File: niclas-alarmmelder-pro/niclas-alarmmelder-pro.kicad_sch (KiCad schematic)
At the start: 16 parts, among them J1 DIN-5_180degree, SW1 SW_SPST, U1 MOUDLE-SEEEDUINO-XIAO-ESP32C3, U2 TME-0503S

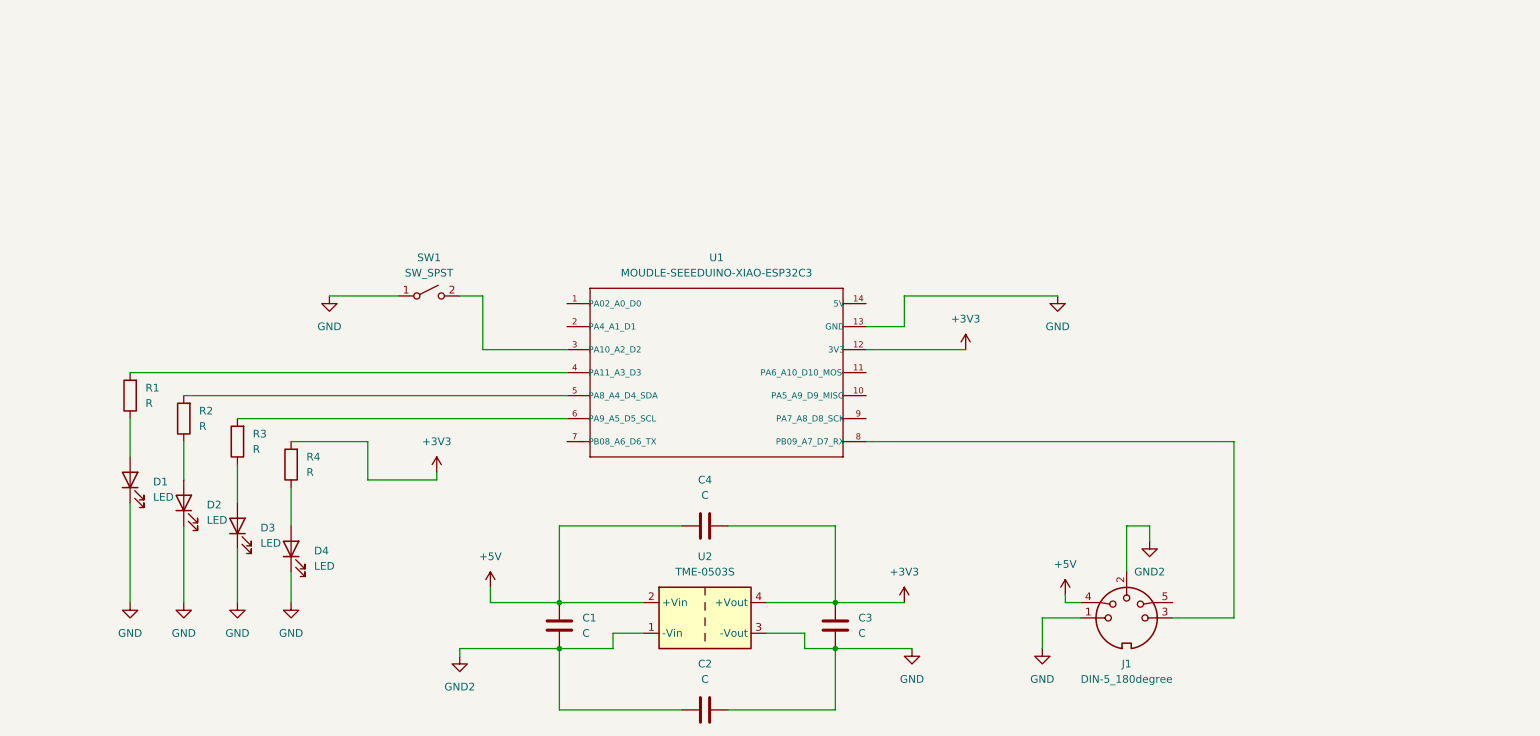
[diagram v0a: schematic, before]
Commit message: release ready
Sollte so funktionieren, eine Schraube mag oder mag nicht accessible sein je nach Schalter aber idc worst case reichen auch 2
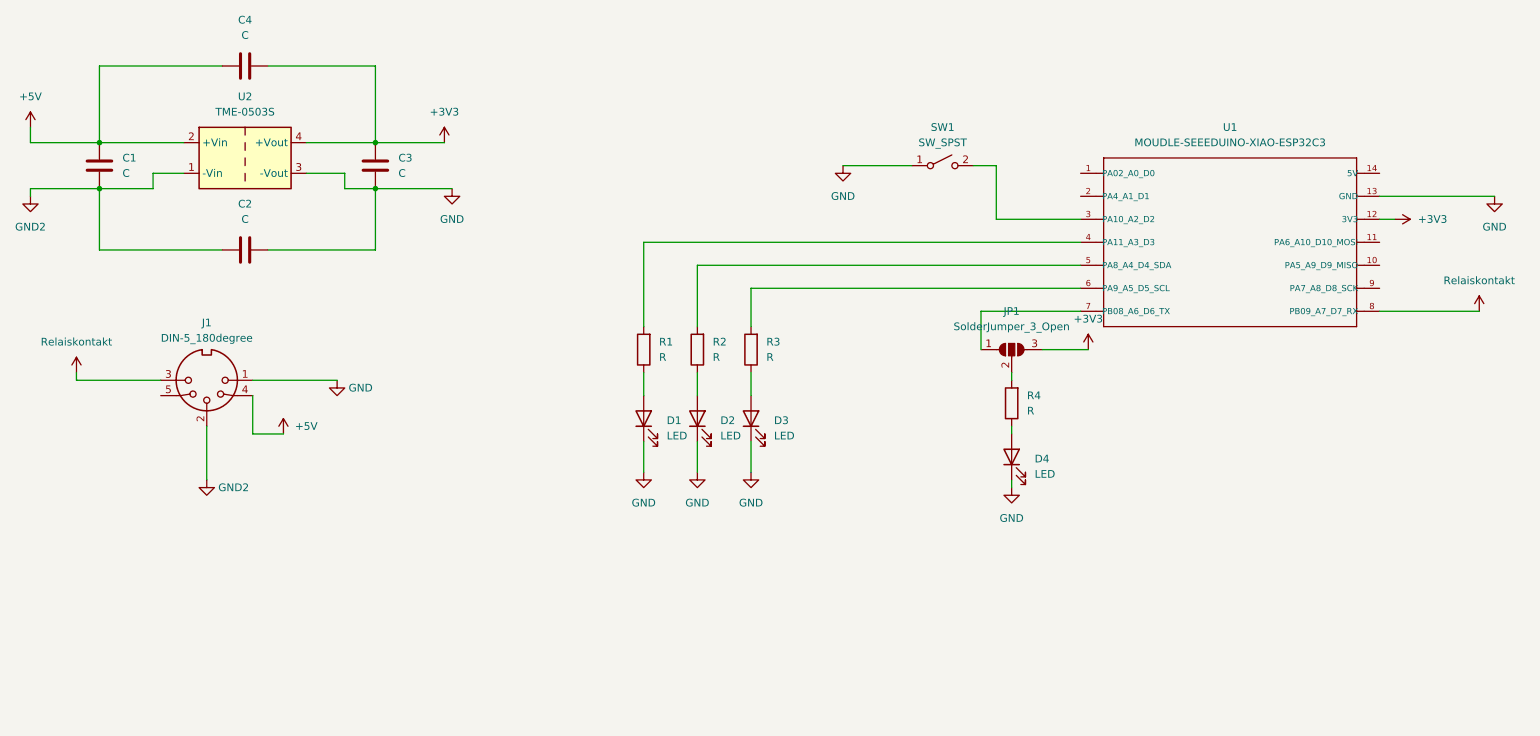
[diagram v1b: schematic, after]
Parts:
- added JP1: SolderJumper_3_Open, Jumper:SolderJumper-3_P2.0mm_Open_TrianglePad1.0x1.5mm_NumberLabels, symbol Jumper:SolderJumper_3_Open
- U1: footprint MOUDLE14P-SMD-2.54-21X17.8MM -> Seeeduino xiao ESP32C3 KiCAD Library:MOUDLE14P-SMD-2.54-21X17.8MM
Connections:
- net +3V3: now also JP1.3 (B); no longer R4.2
- net at U1.7 (PB08_A6_D6_TX): now also JP1.1 (A)
- net Relaiskontakt: now reaches J1.3, U1.8 (PB09_A7_D7_RX)
- new net: JP1.2 (C), R4.2
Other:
- moved on the sheet: C1, C2, C3, C4, D1, D2, D3, D4, J1, R1, R2, R3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
